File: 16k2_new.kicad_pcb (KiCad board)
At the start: 4 copper layers, 160 x 160 mm, 23 parts, among them J1 MUX POTS, J4 To controller board, J5 MUX SIG

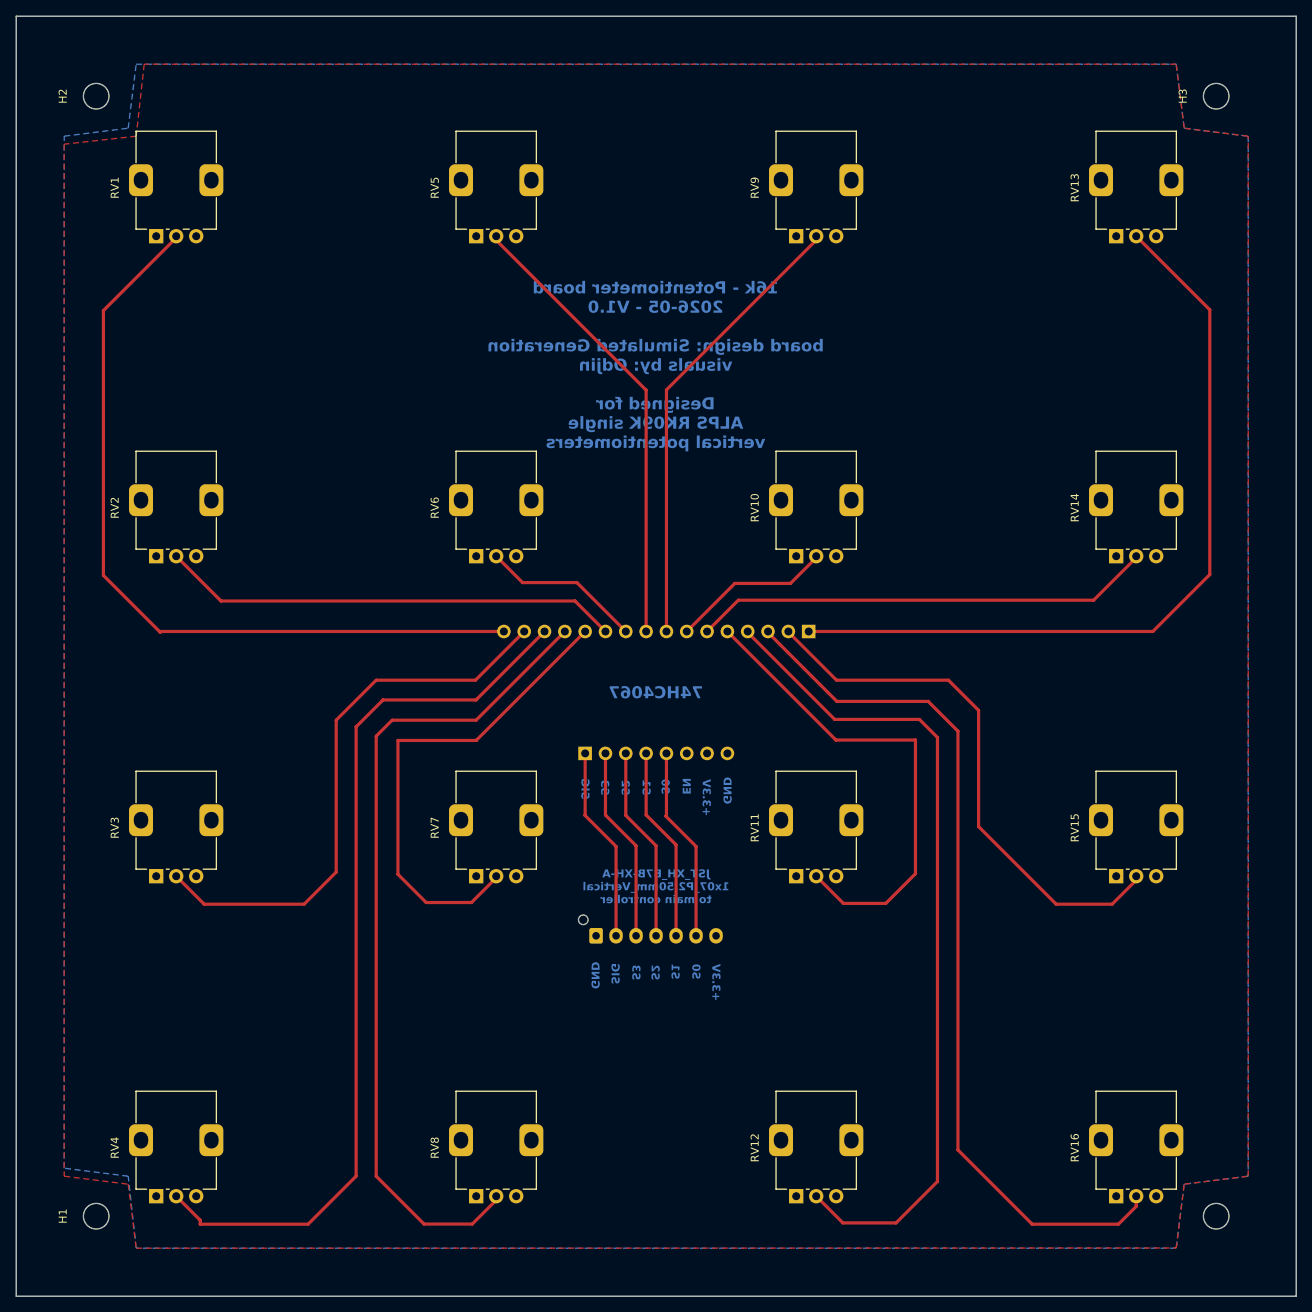
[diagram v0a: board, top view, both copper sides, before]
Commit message: Adds MIT licence
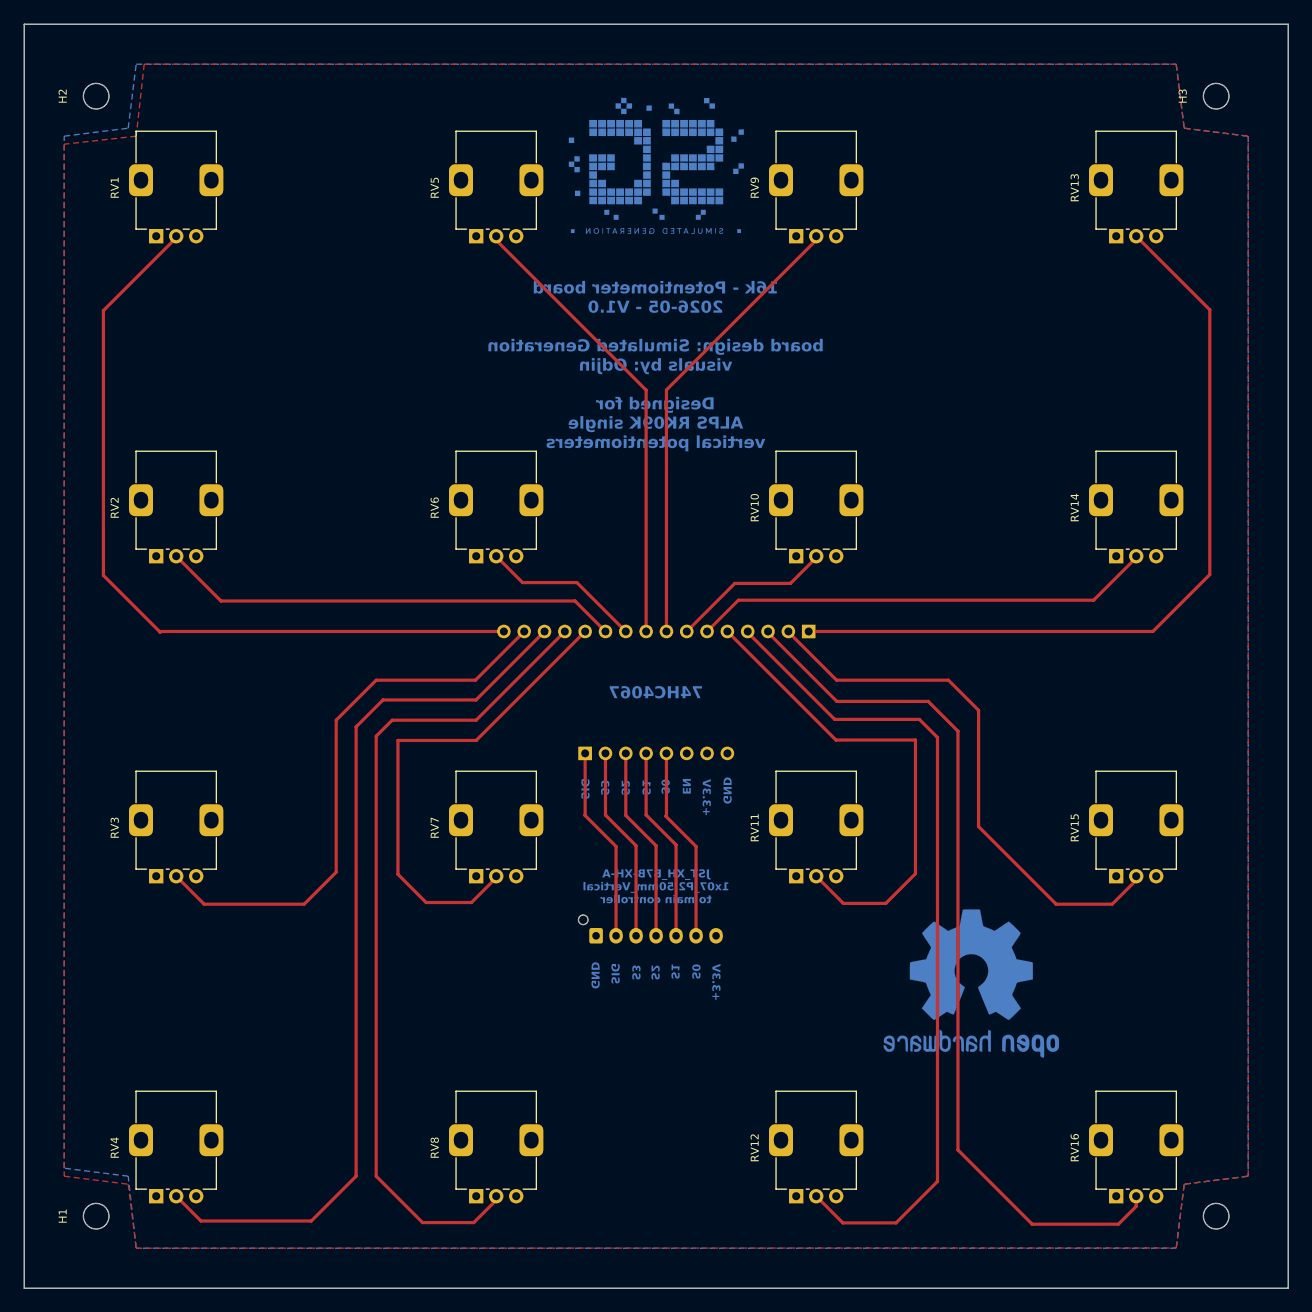
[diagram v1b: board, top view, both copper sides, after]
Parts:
- added G***: LOGO, Custom:logoSG, B.Cu at (100.1, 38.8)
- added REF**: OSHW-Logo2_24.3x20mm_Copper, Symbol:OSHW-Logo2_24.3x20mm_Copper, B.Cu at (139.4, 140.9)
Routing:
- net /K04: track 111.4 -> 110.8 mm
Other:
- board size 160 x 160 mm -> 158 x 158 mm
